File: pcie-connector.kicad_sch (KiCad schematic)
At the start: 6 parts, among them J10 PCB-Edge_PCIexpress_x8, SW1 CVS-03B

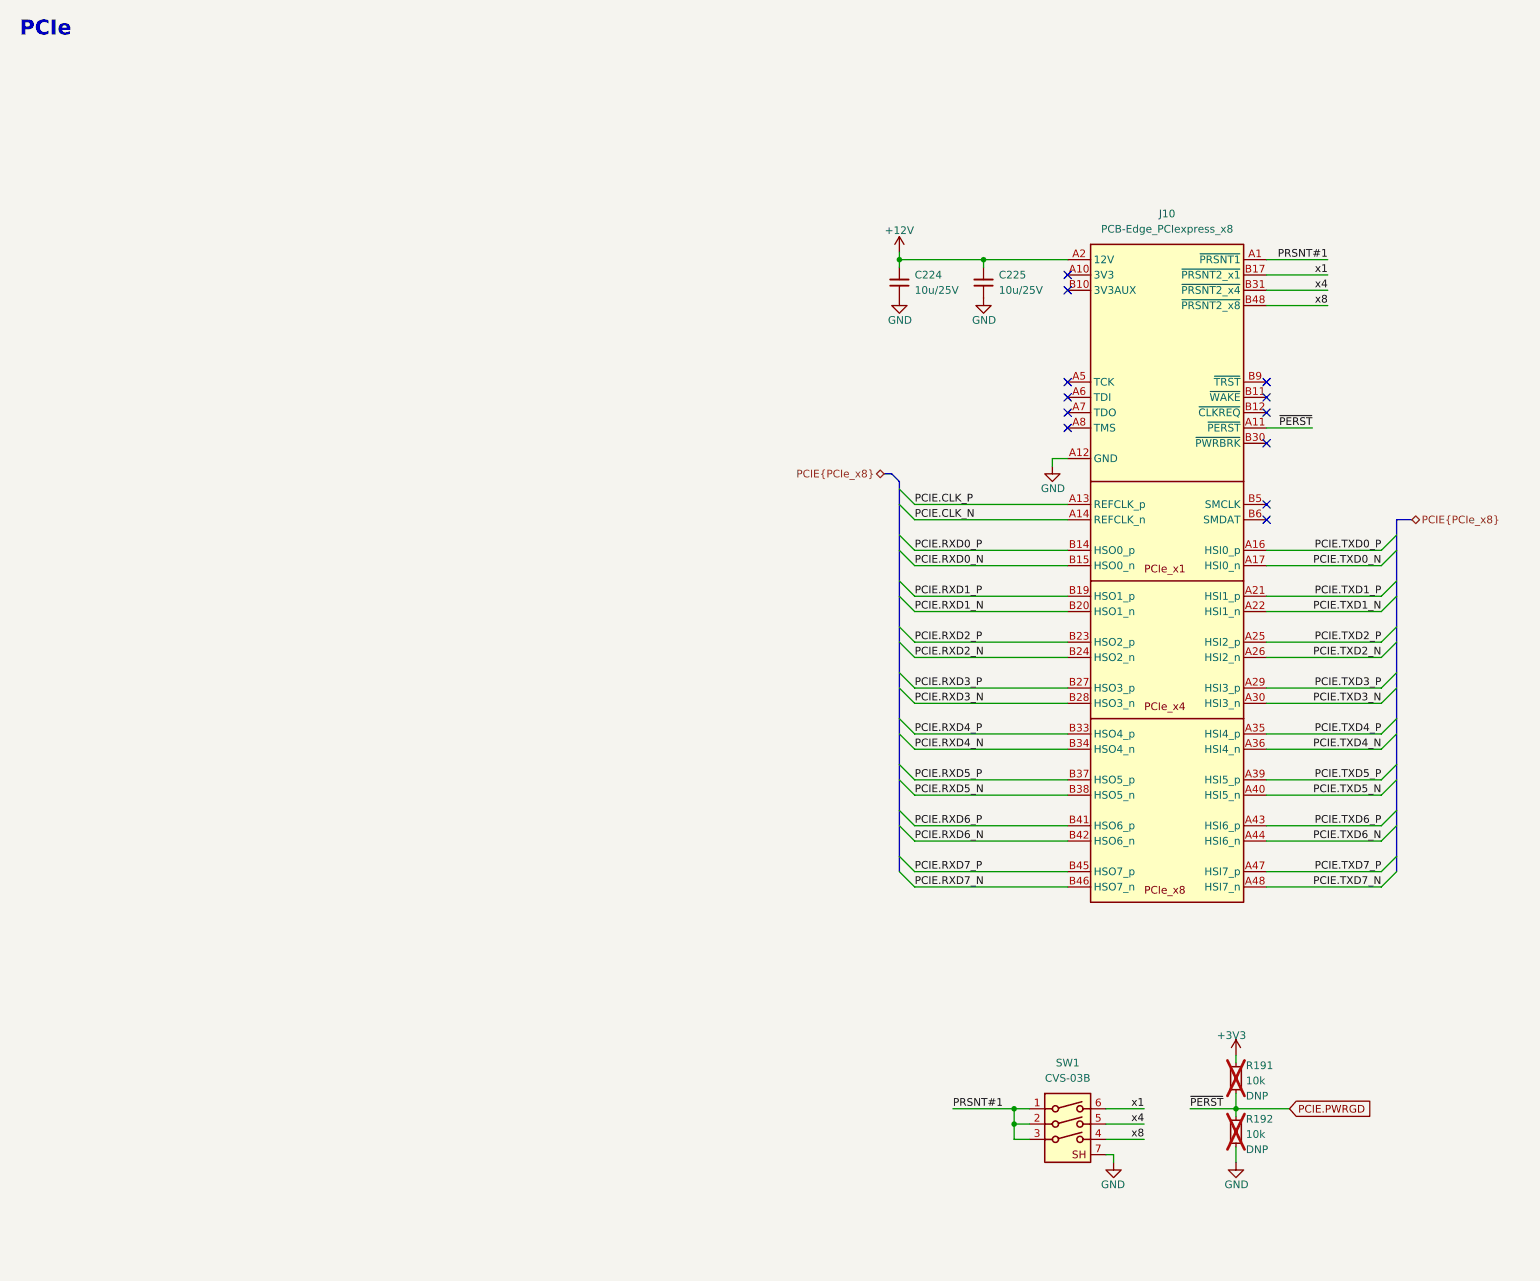
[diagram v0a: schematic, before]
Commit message: [#68016] Clean-up the schematic
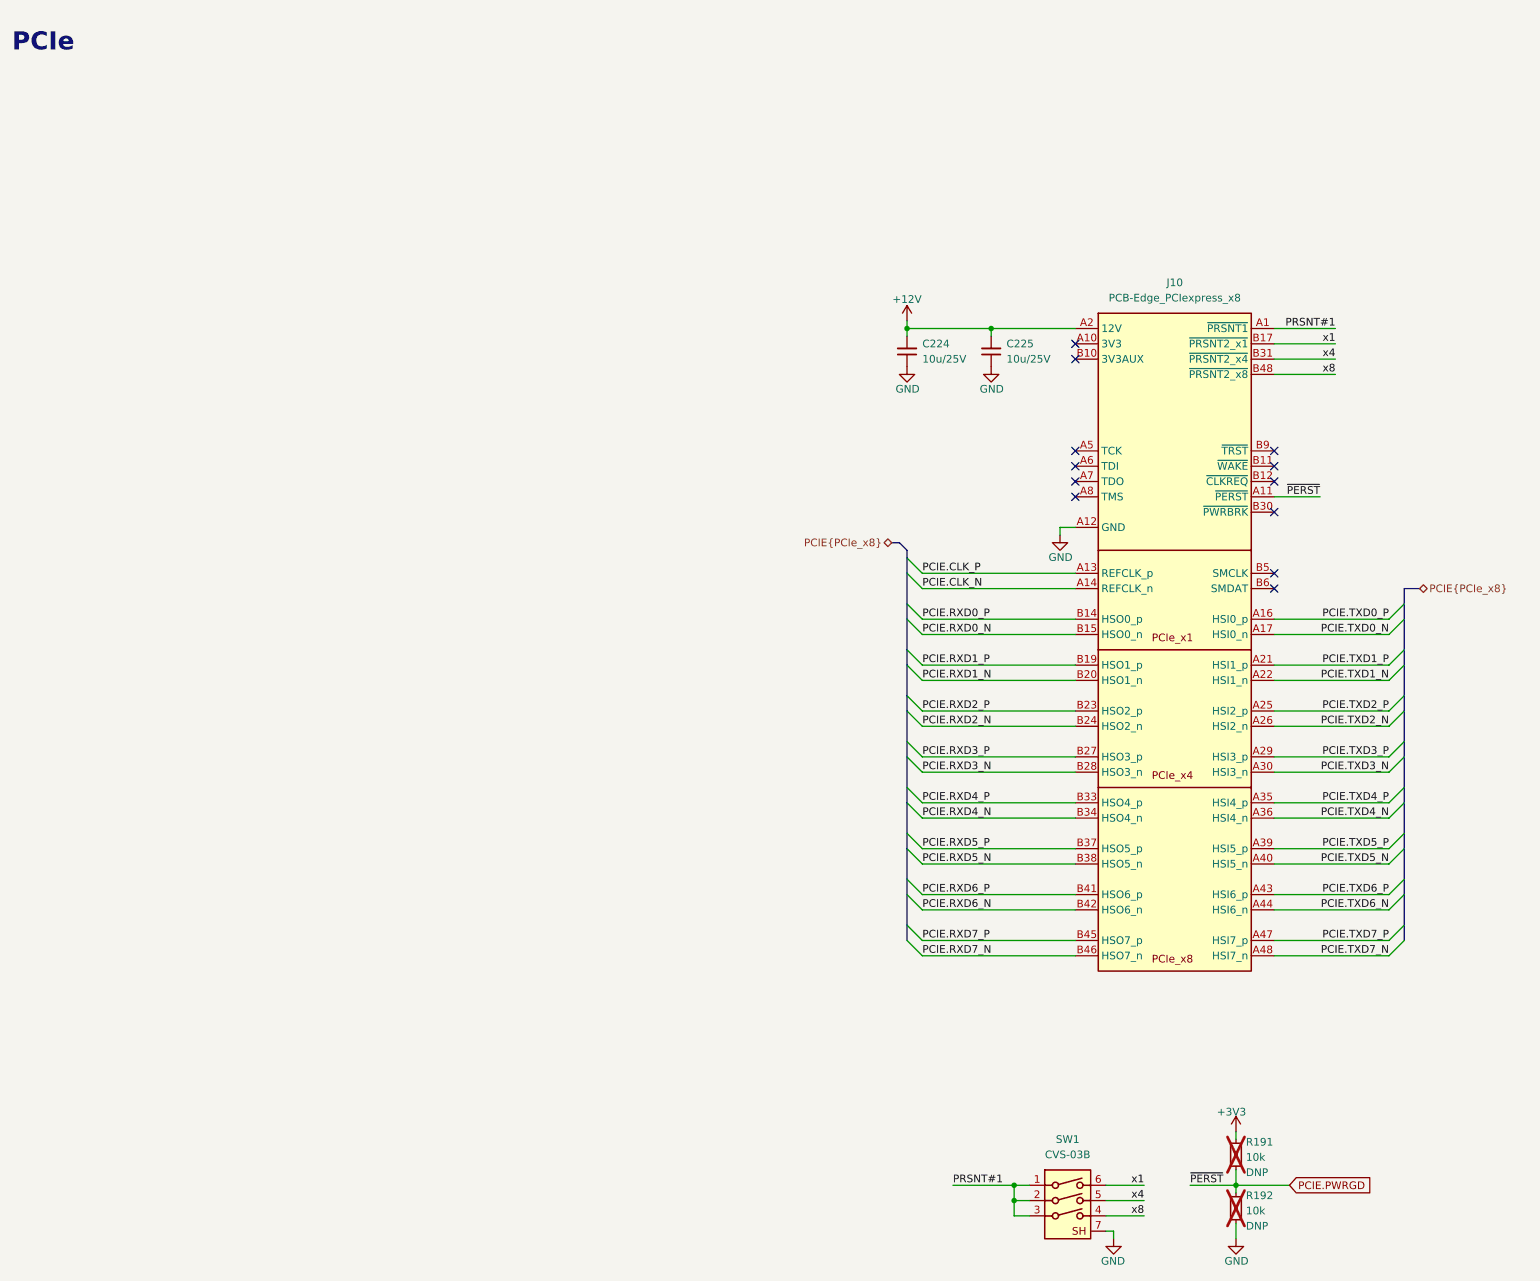
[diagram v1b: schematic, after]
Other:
- moved on the sheet: C224, C225, J10, R191, R192, SW1
